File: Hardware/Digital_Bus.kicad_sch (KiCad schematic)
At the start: 0 parts

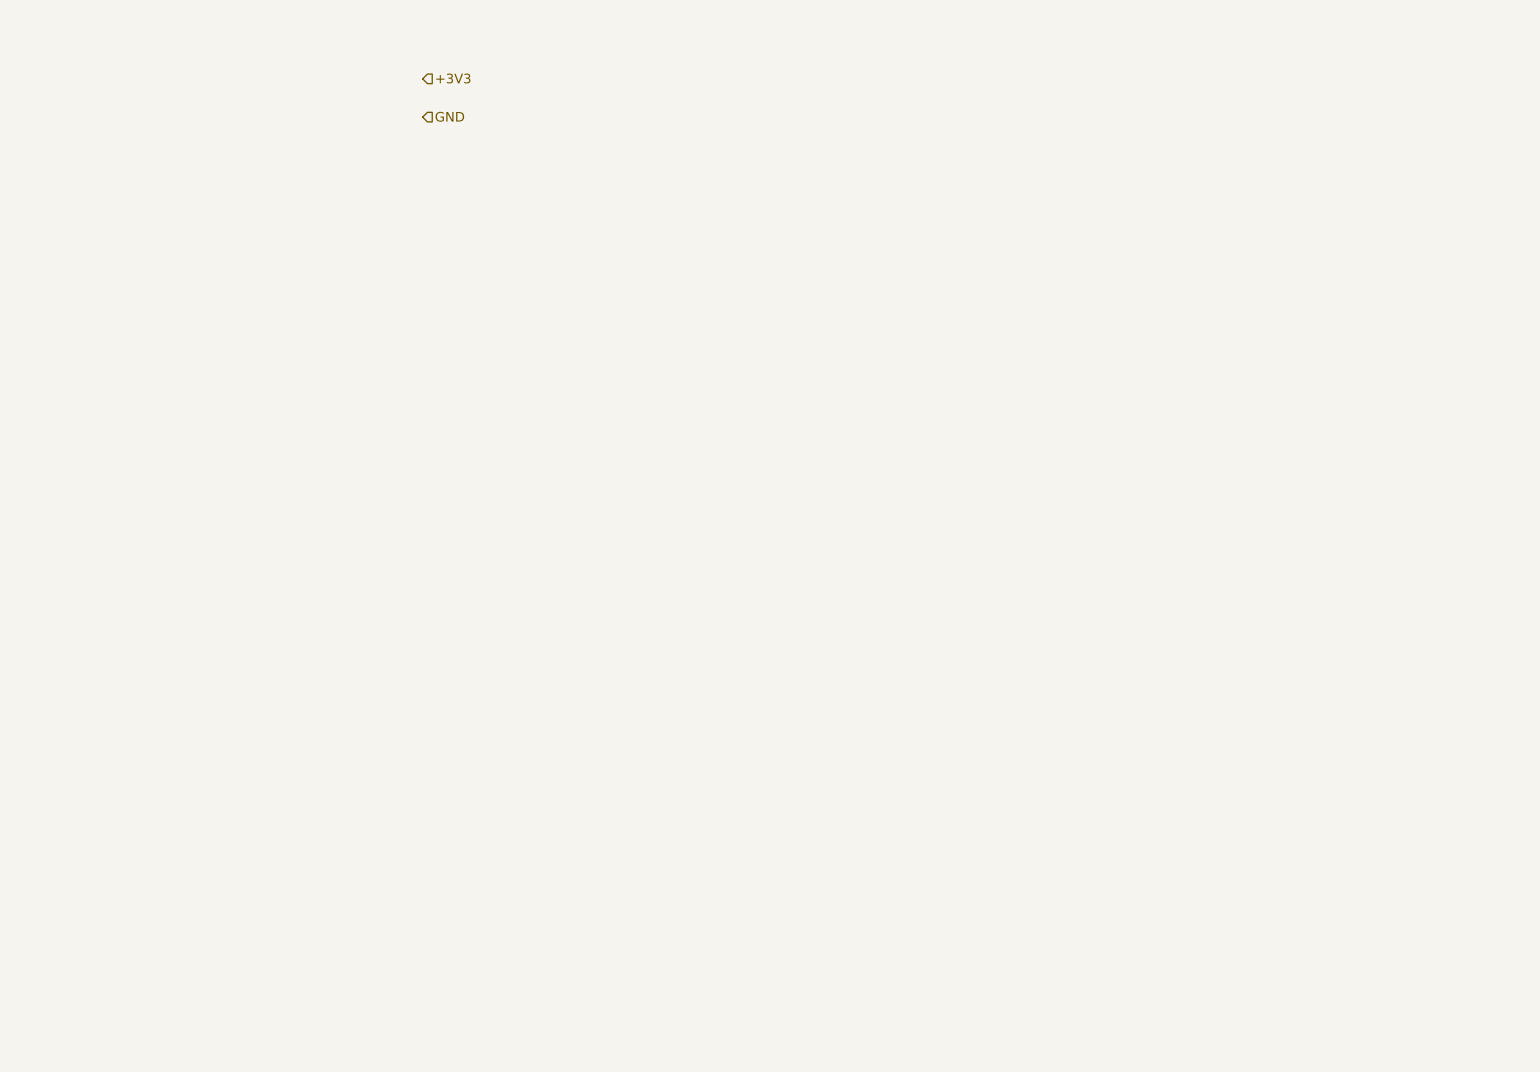
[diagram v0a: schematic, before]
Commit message: Major Updates to Schematic
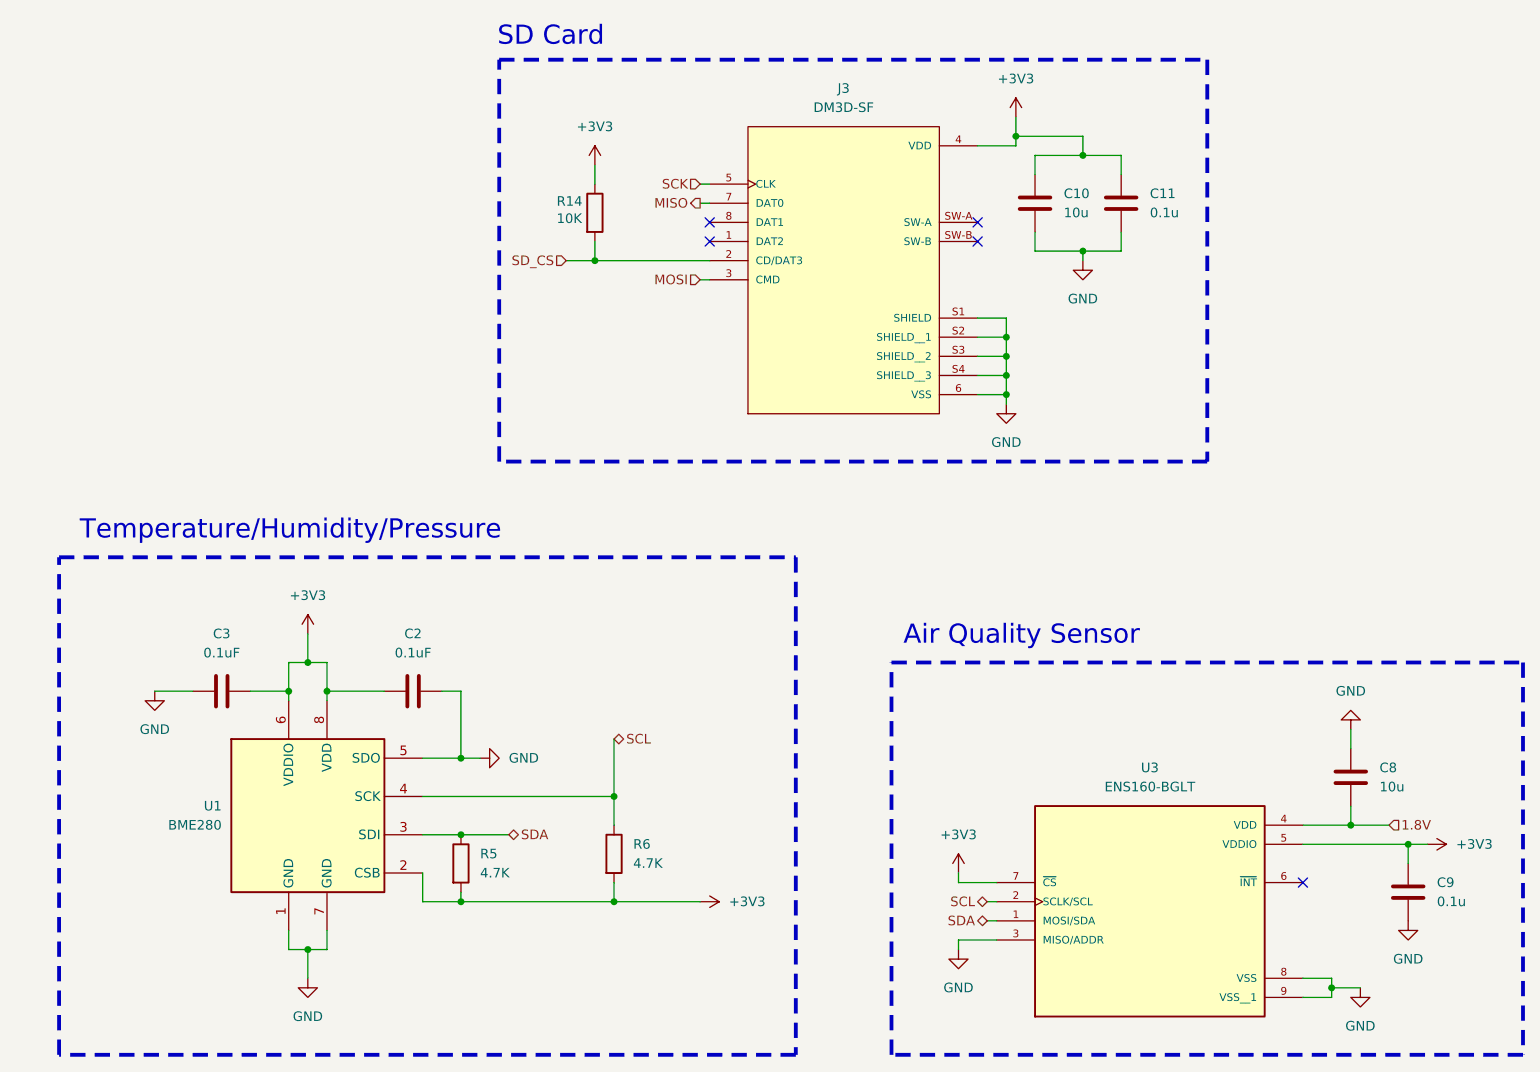
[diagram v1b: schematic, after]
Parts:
- added C10, C8: 10u, symbol Device:C
- added C11, C9: 0.1u, symbol Device:C
- added C2, C3: 0.1uF, symbol Device:C
- added J3: DM3D-SF, Micro_SD_Card:HRS_DM3D-SF, symbol DM3D-SF:DM3D-SF
- added R14: 10K, symbol Device:R
- added R5, R6: 4.7K, symbol Device:R
- added U1: BME280, Package_LGA:Bosch_LGA-8_2.5x2.5mm_P0.65mm_ClockwisePinNumbering, symbol Sensor:BME280
- added U3: ENS160-BGLT, Custom_Sensors:XDCR_ENS160-BGLT, symbol ENS160-BGLT:ENS160-BGLT
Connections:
- net +3V3: now also C10.1, C11.1, C2.1, C3.1, C9.1, J3.4 (VDD), R14.1, R5.2, R6.2, U1.2 (CSB), U1.6 (VDDIO), U1.8 (VDD), U3.5 (VDDIO), U3.7 (~{CS})
- net GND: now also C10.2, C11.2, C2.2, C3.2, C8.1, C9.2, J3.6 (VSS), J3.S1 (SHIELD), J3.S2 (SHIELD__1), J3.S3 (SHIELD__2), J3.S4 (SHIELD__3), U1.1 (GND), U1.5 (SDO), U1.7 (GND), U3.3 (MISO/ADDR), U3.8 (VSS), U3.9 (VSS__1)
- new net 1.8V: C8.2, U3.4 (VDD)
- new net MISO: J3.7 (DAT0)
- new net MOSI: J3.3 (CMD)
- new net SCK: J3.5 (CLK)
- new net SCL: R6.1, U1.4 (SCK), U3.2 (SCLK/SCL)
- new net SDA: R5.1, U1.3 (SDI), U3.1 (MOSI/SDA)
- new net SD_CS: J3.2 (CD/DAT3), R14.2
- no-connect marks 0 -> 5
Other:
- note added: "Air Quality Sensor"
- note added: "SD Card"
- note added: "Temperature/Humidity/Pressure"
